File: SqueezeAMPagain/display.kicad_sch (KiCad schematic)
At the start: 2 parts, among them J5 Conn_02x10_Odd_Even, U4 TSOP21xx

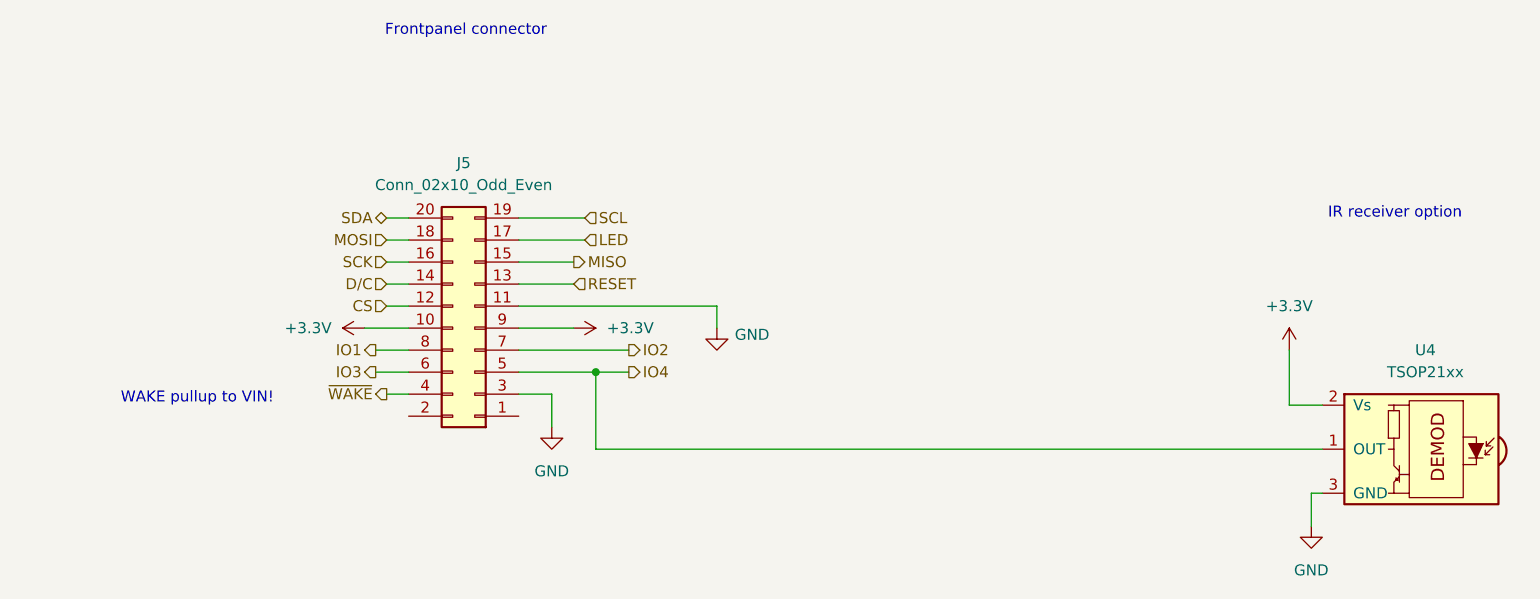
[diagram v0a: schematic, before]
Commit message: v2
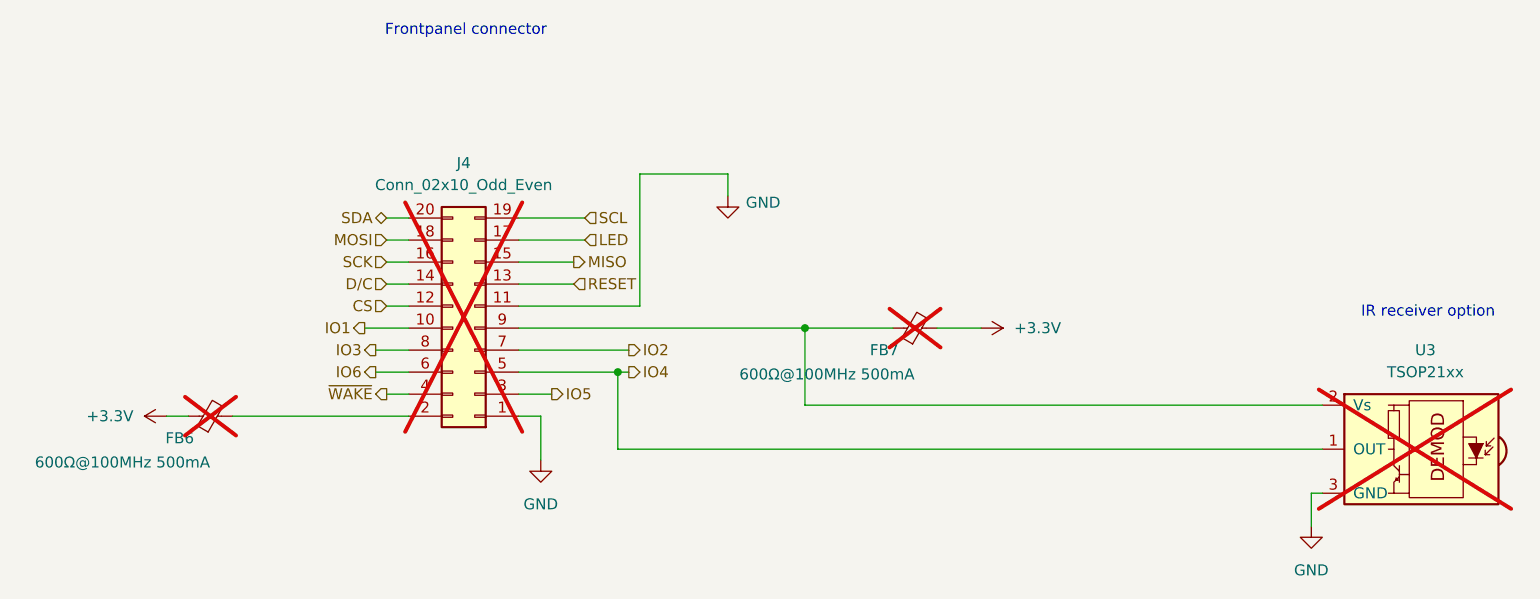
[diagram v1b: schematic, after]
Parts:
- added FB6, FB7: 600Ω@100MHz 500mA, Inductor_SMD:L_0805_2012Metric, symbol Device:FerriteBead_Small
- J4: renamed from J5; now not fitted
- U3: renamed from U4; now not fitted
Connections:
- net +3.3V: now also FB6.1, FB7.2; no longer J4.10 (Pin_10), J4.9 (Pin_9), U3.2 (Vs)
- net GND: now also J4.1 (Pin_1); no longer J4.3 (Pin_3)
- net IO1: now also J4.10 (Pin_10); no longer J4.8 (Pin_8)
- net IO3: now also J4.8 (Pin_8); no longer J4.6 (Pin_6)
- net at J4.2 (Pin_2): now also FB6.2
- new net: FB7.1, J4.9 (Pin_9), U3.2 (Vs)
- new net IO5: J4.3 (Pin_3)
- new net IO6: J4.6 (Pin_6)
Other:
- note removed: "WAKE pullup to VIN!"
